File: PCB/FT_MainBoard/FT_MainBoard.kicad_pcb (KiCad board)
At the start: 2 copper layers, 84 x 53 mm, 49 parts, among them SW1 SW_Push, SW2 SW_SPST

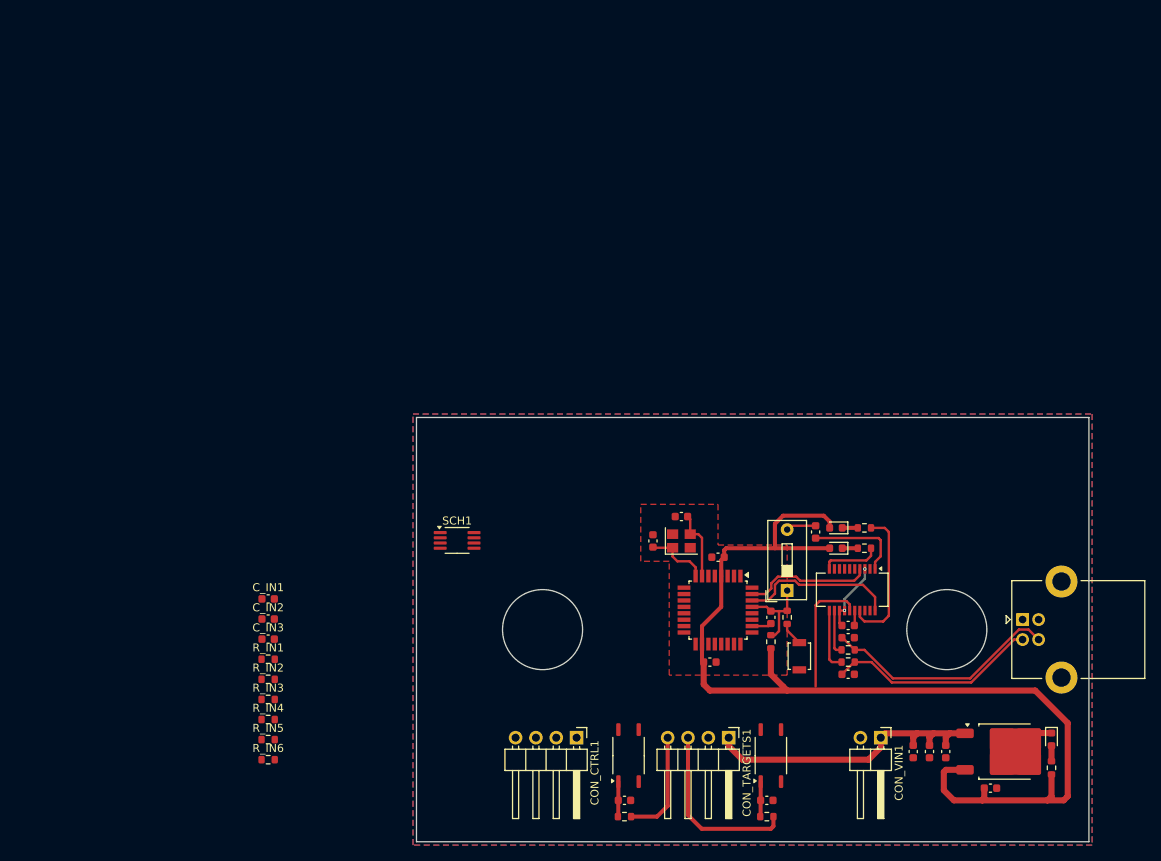
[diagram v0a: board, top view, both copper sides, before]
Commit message: final update
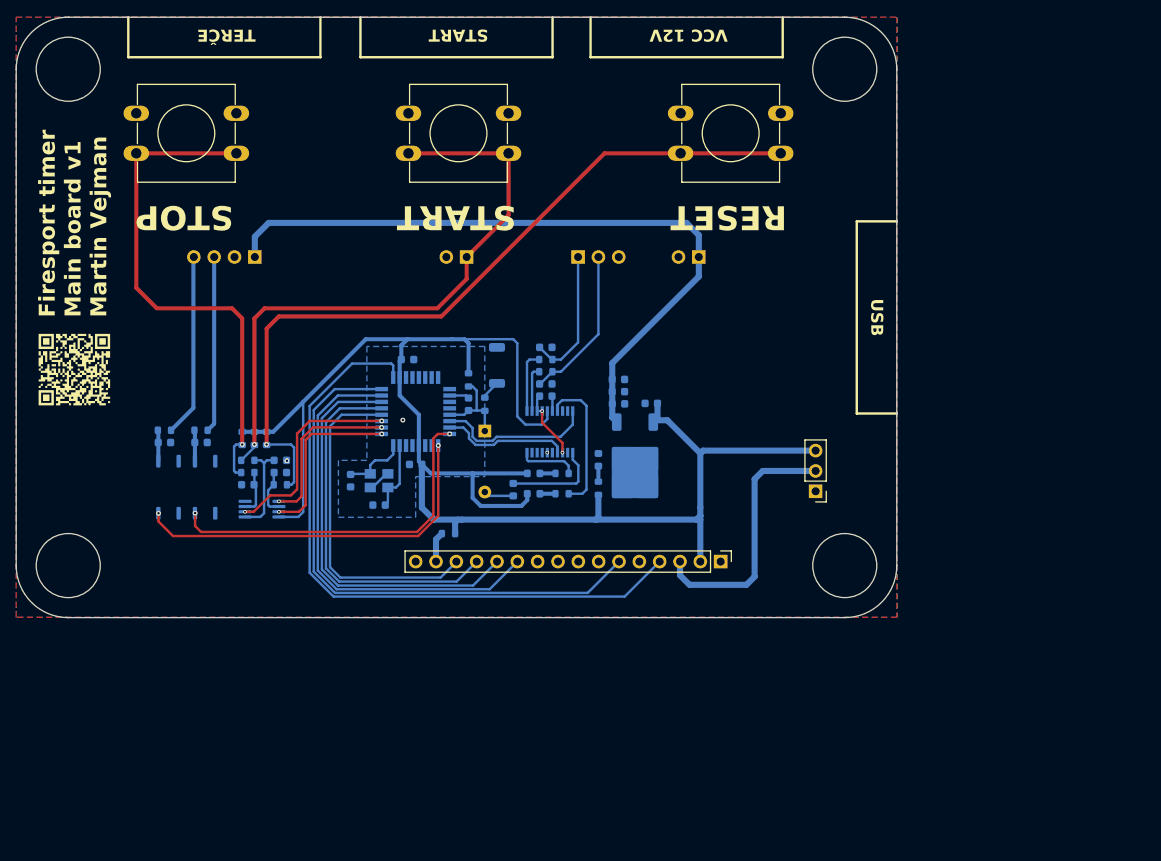
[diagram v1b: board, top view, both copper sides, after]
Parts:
- removed CON_CTRL1: Conn_01x04_Pin, Connector_PinHeader_2.54mm:PinHeader_1x04_P2.54mm_Horizontal
- removed USB1: USB_B, Connector_USB:USB_B_Lumberg_2411_02_Horizontal
- added CON1: Conn_01x02_Pin, custom_components:CON_2_pin, B.Cu at (105.0, 80.0)
- added CON3: Conn_01x03, custom_components:CON_3_pin, B.Cu at (122.7, 80.0)
- added G***: LOGO, custom_components:QR, F.Cu at (57.2, 94.0)
- added HDR1: Conn_01x16_Pin, Connector_PinHeader_2.54mm:PinHeader_1x16_P2.54mm_Vertical, F.Cu at (138.0, 118.0)
- added R1: 200R, Resistor_SMD:R_0603_1608Metric, B.Cu at (104.0, 114.5)
- added RV1: Vishay 64X 10K, Connector_PinHeader_2.54mm:PinHeader_1x03_P2.54mm_Vertical, F.Cu at (149.9, 109.2)
- added SW1: SW_Push, Button_Switch_THT:SW_PUSH-12mm, F.Cu at (99.0, 62.0)
- added SW2: SW_Push, Button_Switch_THT:SW_PUSH-12mm, F.Cu at (65.0, 62.0)
- added SW3: SW_Push, Button_Switch_THT:SW_PUSH-12mm, F.Cu at (133.0, 62.0)
- C1: renamed from C_MCU1; moved to B.Cu
- C10: renamed from C_IN3; moved to B.Cu
- C11: renamed from C_VIN1; moved to B.Cu
- C12: renamed from C_VIN2; moved to B.Cu
- C13: renamed from C_VIN3; moved to B.Cu
- C14: renamed from C_OPTL1; moved to B.Cu
- C15: renamed from C_OPTR1; moved to B.Cu
- C16: renamed from C_RES1; moved to B.Cu
- C17: renamed from C_LREG1; moved to B.Cu
- C18: renamed from C_RES2; moved to B.Cu
- C2: renamed from C_MCU2; moved to B.Cu
- C3: renamed from C_MCU_OSC1; moved to B.Cu
- C4: renamed from C_MCU_OSC2; moved to B.Cu
- C5: renamed from C_USB1; moved to B.Cu
- C6: renamed from C_USB2; moved to B.Cu
- C7: renamed from C_USB3; moved to B.Cu
- C8: renamed from C_IN1; moved to B.Cu
- C9: renamed from C_IN2; moved to B.Cu
- CON4: renamed from CON_VIN1; footprint Connector_PinHeader_2.54mm:PinHeader_1x02_P2.54mm_Horizontal -> custom_components:CON_2_pin; moved to B.Cu
- CON5: renamed from CON_TARGETS1; footprint Connector_PinHeader_2.54mm:PinHeader_1x04_P2.54mm_Horizontal -> custom_components:CON_4_pin; moved to B.Cu
- IC1: renamed from MCU1; value ATmega328PB-A -> ATmega328PB-AU; moved to B.Cu
- IC2: renamed from UART-USB1; value FT231XS -> FT231XS-R; moved to B.Cu
- IC3: renamed from SCH1; moved to B.Cu
- IC4: renamed from LREG1; value LM78M05_TO252 -> L78M05ABDT-TR; moved to B.Cu
- LED1: renamed from LED_RX1; moved to B.Cu
- LED2: renamed from LED_TX1; moved to B.Cu
- LED3: renamed from LED_PWR1; moved to B.Cu
- OPT1: renamed from OPTL1; moved to B.Cu
- OPT2: renamed from OPTR1; moved to B.Cu
- OSC1: renamed from OSC_MCU1; moved to B.Cu
- R10: renamed from R_IN2; moved to B.Cu
- R11: renamed from R_IN3; moved to B.Cu
- R12: renamed from R_RES1; moved to B.Cu
- R13: renamed from RL1; moved to B.Cu
- R14: renamed from RR1; moved to B.Cu
- R15: renamed from R_RES2; moved to B.Cu
- R16: renamed from R1; moved to B.Cu
- R2, R3: moved to B.Cu
- R4: renamed from R_USB1; moved to B.Cu
- R5: renamed from R_USB2; moved to B.Cu
- R6: renamed from R_IN4; moved to B.Cu
- R7: renamed from R_IN5; moved to B.Cu
- R8: renamed from R_IN6; moved to B.Cu
- R9: renamed from R_IN1; moved to B.Cu
- SW4: renamed from SW1; footprint Button_Switch_SMD:SW_SPST_B3U-1000P -> custom_components:switch; moved to B.Cu
- SW5: renamed from SW2; moved to B.Cu
- moved CON5 87.0 mm to (76.0, 80.0), turned to 90 degrees
- moved R13 85.6 mm to (73.1, 101.6)
- moved C14 83.6 mm to (73.1, 103.1)
- moved OPT1 78.2 mm to (73.6, 108.7), turned to -90 degrees
- moved R14 75.0 mm to (68.5, 101.6)
- moved C15 72.8 mm to (68.5, 103.1)
- moved OPT2 66.5 mm to (69.0, 108.7), turned to -90 degrees
- moved R16 66.5 mm to (122.7, 108.8)
- moved LED3 66.5 mm to (122.7, 105.3)
- moved CON4 64.7 mm to (134.0, 80.0), turned to 90 degrees
- moved C17 64.1 mm to (129.3, 98.2), turned to 180 degrees
- moved C13 59.6 mm to (125.2, 98.3), turned to 0 degrees
- moved C12 59.4 mm to (125.2, 96.8), turned to 0 degrees
- moved C11 59.3 mm to (125.2, 95.2), turned to 0 degrees
- moved IC4 58.7 mm to (127.3, 105.6), turned to -90 degrees
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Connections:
- IC1 pad 10: RESET -> STOP
- IC1 pad 11: GND -> RESET
- IC1 pad 12: DISPLAY_RS -> DISPLAY_D3
- IC1 pad 13: DISPLAY_EN -> DISPLAY_D2
- IC1 pad 14: DISPLAY_D3 -> DISPLAY_D1
- IC1 pad 15: DISPLAY_D2 -> DISPLAY_D0
- IC1 pad 16: DISPLAY_D1 -> DISPLAY_EN
- IC1 pad 17: DISPLAY_D0 -> DISPLAY_RS
- IC1 pad 2: START -> GND
- IC1 pad 9: STOP -> START
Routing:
- net Net-(R11-Pad1): track 0.00 -> 96.8 mm, vias 0 -> 1
- net DISPLAY_RS: track 0.00 -> 81.8 mm
- net Net-(CON1-Pin_1): track 0.00 -> 77.3 mm, vias 0 -> 1
- net DISPLAY_EN: track 0.00 -> 70.6 mm
- net Net-(R10-Pad1): track 0.00 -> 65.1 mm, vias 0 -> 1
- net DISPLAY_D0: track 0.00 -> 55.7 mm
- net +5V: track 147.3 -> 202.1 mm
- net DISPLAY_D1: track 0.00 -> 51.2 mm
- net +12V: track 38.5 -> 87.4 mm
- net OPTR: track 0.00 -> 46.6 mm, vias 0 -> 2
- net DISPLAY_D2: track 0.00 -> 46.5 mm
- net OPTL: track 0.00 -> 44.4 mm, vias 0 -> 2
- net DISPLAY_D3: track 0.00 -> 41.8 mm
- net Net-(HDR1-Pin_3): track 0.00 -> 32.2 mm
- net RESET: track 0.00 -> 25.9 mm, vias 0 -> 2
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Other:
- board size 84 x 53 mm -> 110 x 75 mm
- board text added: "+"
- board text added: "+5V"
- board text added: "-"
- board text added: "D+"
- board text added: "D-"
- board text added: "Firesport timer Main board v1 Martin Vejman"
- board text added: "L"
- board text added: "MCU RESET"
- board text added: "P"
- board text added: "PROGRAM"
- board text added: "Q"
- board text added: "RESET"
- board text added: "START"
- board text added: "STOP"
- board text added: "TERČE"
- board text added: "TRIM"
- board text added: "USB"
- board text added: "VCC 12V"
